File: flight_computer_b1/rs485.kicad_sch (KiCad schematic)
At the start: 1 part, among them U7 MIC94161YCS-TR

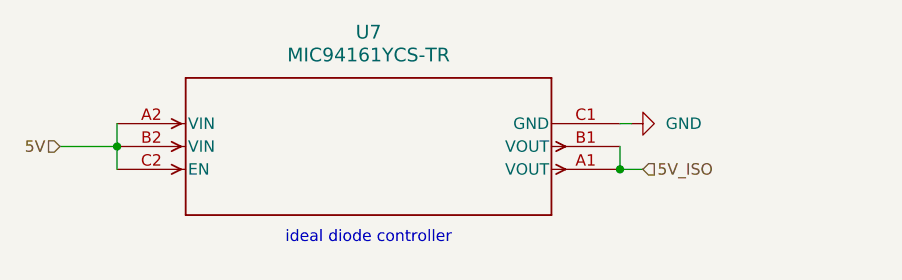
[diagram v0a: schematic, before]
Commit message: flight computer updates
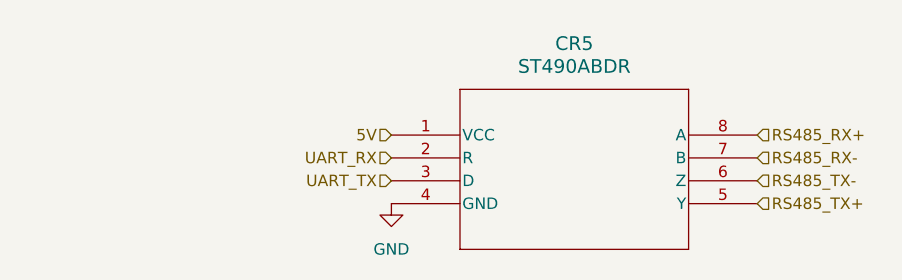
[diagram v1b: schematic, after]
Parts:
- removed U7: MIC94161YCS-TR, avi_lib:MIC94161YCS_TR, symbol avi_lib:MIC94161YCS-TR
- added CR5: ST490ABDR, SO-8_STM, symbol avi_lib:ST490ABDR
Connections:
- net 5V: now also CR5.1 (VCC)
- net GND: now also CR5.4 (GND)
- new net RS485_RX+: CR5.8 (A)
- new net RS485_RX-: CR5.7 (B)
- new net RS485_TX+: CR5.5 (Y)
- new net RS485_TX-: CR5.6 (Z)
- new net UART_RX: CR5.2 (R)
- new net UART_TX: CR5.3 (D)
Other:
- note removed: "ideal diode controller"
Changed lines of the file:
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@@
 	(generator_version "9.0")
 	(paper "A4")
-	(text "ideal diode controller"
-		(exclude_from_sim no)
-		(at 134.62 102.87 0)
-		(effects
-			(font
-				(size 1.27 1.27)
-			)
-		)
-	)
-	(junction
-		(at 106.68 92.71)
-		(diameter 0)
-		(color 0 0 0 0)
-	)
-	(junction
-		(at 162.56 95.25)
-		(diameter 0)
-		(color 0 0 0 0)
-	)
-	(wire
-		(pts
-			(xy 162.56 92.71) (xy 162.56 95.25)
-		)
-		(stroke
-			(width 0)
-			(type default)
-		)
-	)
-	(wire
-		(pts
-			(xy 106.68 92.71) (xy 106.68 95.25)
-		)
-		(stroke
-			(width 0)
-			(type default)
-		)
-	)
-	(wire
-		(pts
-			(xy 162.56 95.25) (xy 165.1 95.25)
-		)
-		(stroke
-			(width 0)
-			(type default)
-		)
-	)
-	(wire
-		(pts
-			(xy 106.68 90.17) (xy 106.68 92.71)
-		)
-		(stroke
-			(width 0)
-			(type default)
-		)
-	)
-	(wire
-		(pts
-			(xy 100.33 92.71) (xy 106.68 92.71)
-		)
-		(stroke
-			(width 0)
-			(type default)
-		)
-	)
-	(wire
-		(pts
-			(xy 163.83 90.17) (xy 162.56 90.17)
-		)
-		(stroke
-			(width 0)
-			(type default)
+	(hierarchical_label "UART_TX"
+		(shape input)
+		(at 137.16 96.52 180)
+		(effects
+			(font
+				(size 1.27 1.27)
+			)
+			(justify right)
+		)
+	)
+	(hierarchical_label "UART_RX"
+		(shape input)
+		(at 137.16 93.98 180)
+		(effects
+			(font
+				(size 1.27 1.27)
+			)
+			(justify right)
+		)
+	)
+	(hierarchical_label "RS485_TX+"
+		(shape input)
+		(at 177.8 99.06 0)
+		(effects
+			(font
+				(size 1.27 1.27)
+			)
+			(justify left)
+		)
+	)
+	(hierarchical_label "RS485_TX-"
+		(shape input)
+		(at 177.8 96.52 0)
+		(effects
+			(font
+				(size 1.27 1.27)
+			)
+			(justify left)
+		)
+	)
+	(hierarchical_label "RS485_RX+"
+		(shape input)
+		(at 177.8 91.44 0)
+		(effects
+			(font
+				(size 1.27 1.27)
+			)
+			(justify left)
+		)
+	)
+	(hierarchical_label "RS485_RX-"
+		(shape input)
+		(at 177.8 93.98 0)
+		(effects
+			(font
+				(size 1.27 1.27)
+			)
+			(justify left)
 		)
 	)
 	(hierarchical_label "5V"
 		(shape input)
-		(at 100.33 92.71 180)
+		(at 137.16 91.44 180)
 		(effects
 			(font
@@
 			)
 			(justify right)
-		)
-	)
-	(hierarchical_label "5V_ISO"
-		(shape input)
-		(at 165.1 95.25 0)
-		(effects
-			(font
-				(size 1.27 1.27)
-			)
-			(justify left)
 		)
 	)
 	(symbol
 		(lib_id "power:GND")
-		(at 163.83 90.17 90)
+		(at 137.16 99.06 0)
 		(unit 1)
 		(exclude_from_sim no)
@@
 		(dnp no)
 		(fields_autoplaced yes)
-		(property "Reference" "#PWR055"
-			(at 170.18 90.17 0)
+		(property "Reference" "#PWR056"
+			(at 137.16 105.41 0)
 			(effects
 				(font
@@
 		)
 		(property "Value" "GND"
-			(at 167.64 90.1699 90)
-			(effects
-				(font
-					(size 1.27 1.27)
-				)
-				(justify right)
+			(at 137.16 104.14 0)
+			(effects
+				(font
+					(size 1.27 1.27)
+				)
 			)
 		)
 		(property "Footprint" ""
-			(at 163.83 90.17 0)
+			(at 137.16 99.06 0)
 			(effects
 				(font
@@
 		)
 		(property "Datasheet" ""
-			(at 163.83 90.17 0)
+			(at 137.16 99.06 0)
 			(effects
 				(font
@@
 		)
 		(property "Description" "Power symbol creates a global label with name \"GND\" , ground"
-			(at 163.83 90.17 0)
+			(at 137.16 99.06 0)
 			(effects
 				(font
@@
 		)
 		(instances
-			(project "flight_computer"
-				(path "/b71a7b79-cdb5-4e38-a72c-0daaa3474f05/4c75cebc-ee68-4292-a47b-c723457cf341"
-					(reference "#PWR055")
+			(project ""
+				(path "/b71a7b79-cdb5-4e38-a72c-0daaa3474f05/7fe62967-9424-47cf-ae6f-da5e7ca252e6"
+					(reference "#PWR056")
 					(unit 1)
 				)
@@
 	)
 	(symbol
-		(lib_id "avi_lib:MIC94161YCS-TR")
-		(at 106.68 90.17 0)
+		(lib_id "avi_lib:ST490ABDR")
+		(at 137.16 91.44 0)
 		(unit 1)
 		(exclude_from_sim no)
@@
 		(dnp no)
 		(fields_autoplaced yes)
-		(property "Reference" "U7"
-			(at 134.62 80.01 0)
+		(property "Reference" "CR5"
+			(at 157.48 81.28 0)
 			(effects
 				(font
@@
 			)
 		)
-		(property "Value" "MIC94161YCS-TR"
-			(at 134.62 82.55 0)
+		(property "Value" "ST490ABDR"
+			(at 157.48 83.82 0)
 			(effects
 				(font
@@
 			)
 		)
-		(property "Footprint" "avi_lib:MIC94161YCS_TR"
-			(at 106.68 90.17 0)
+		(property "Footprint" "SO-8_STM"
+			(at 137.16 91.44 0)
 			(effects
 				(font
@@
 			)
 		)
-		(property "Datasheet" "MIC94161YCS-TR"
-			(at 106.68 90.17 0)
+		(property "Datasheet" "https://www.st.com/resource/en/datasheet/st490ab.pdf"
+			(at 137.16 91.44 0)
 			(effects
 				(font
@@
 		)
 		(property "Description" ""
-			(at 106.68 90.17 0)
-			(effects
-				(font
-					(size 1.27 1.27)
-				)
-				(hide yes)
-			)
-		)
-		(pin "C1"
-		)
-		(pin "B2"
-		)
-		(pin "C2"
-		)
-		(pin "A1"
-		)
-		(pin "B1"
-		)
-		(pin "A2"
+			(at 137.16 91.44 0)
+			(effects
+				(font
+					(size 1.27 1.27)
+				)
+				(hide yes)
+			)
+		)
+		(pin "8"
+		)
+		(pin "1"
+		)
+		(pin "2"
+		)
+		(pin "4"
+		)
+		(pin "7"
+		)
+		(pin "3"
+		)
+		(pin "6"
+		)
+		(pin "5"
 		)
 		(instances
-			(project "flight_computer"
-				(path "/b71a7b79-cdb5-4e38-a72c-0daaa3474f05/4c75cebc-ee68-4292-a47b-c723457cf341"
-					(reference "U7")
+			(project ""
+				(path "/b71a7b79-cdb5-4e38-a72c-0daaa3474f05/7fe62967-9424-47cf-ae6f-da5e7ca252e6"
+					(reference "CR5")
 					(unit 1)
 				)
